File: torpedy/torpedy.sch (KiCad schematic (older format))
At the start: 45 parts, among them J1 Charger R.C., J10 żółty, J11 zielony, J12 różowy, J13 niebieski, J14 czerwony, J15 brązowy, J16 ekran, J2 step_up - Vin, J3 step_up - Vout, J4 Zasilanie Serwa, J5 Batt HP, J6 RPi I/O, J7 Trigger, J8 biały, J9 szary, Q1 Q_NPN_BCE, Q2 IRL2203N, Q3 Q_NPN_BCE, Q4 IRL2203N, U1 LTV-817, U2 LTV-817, U3 LTV-817, U4 LTV-817

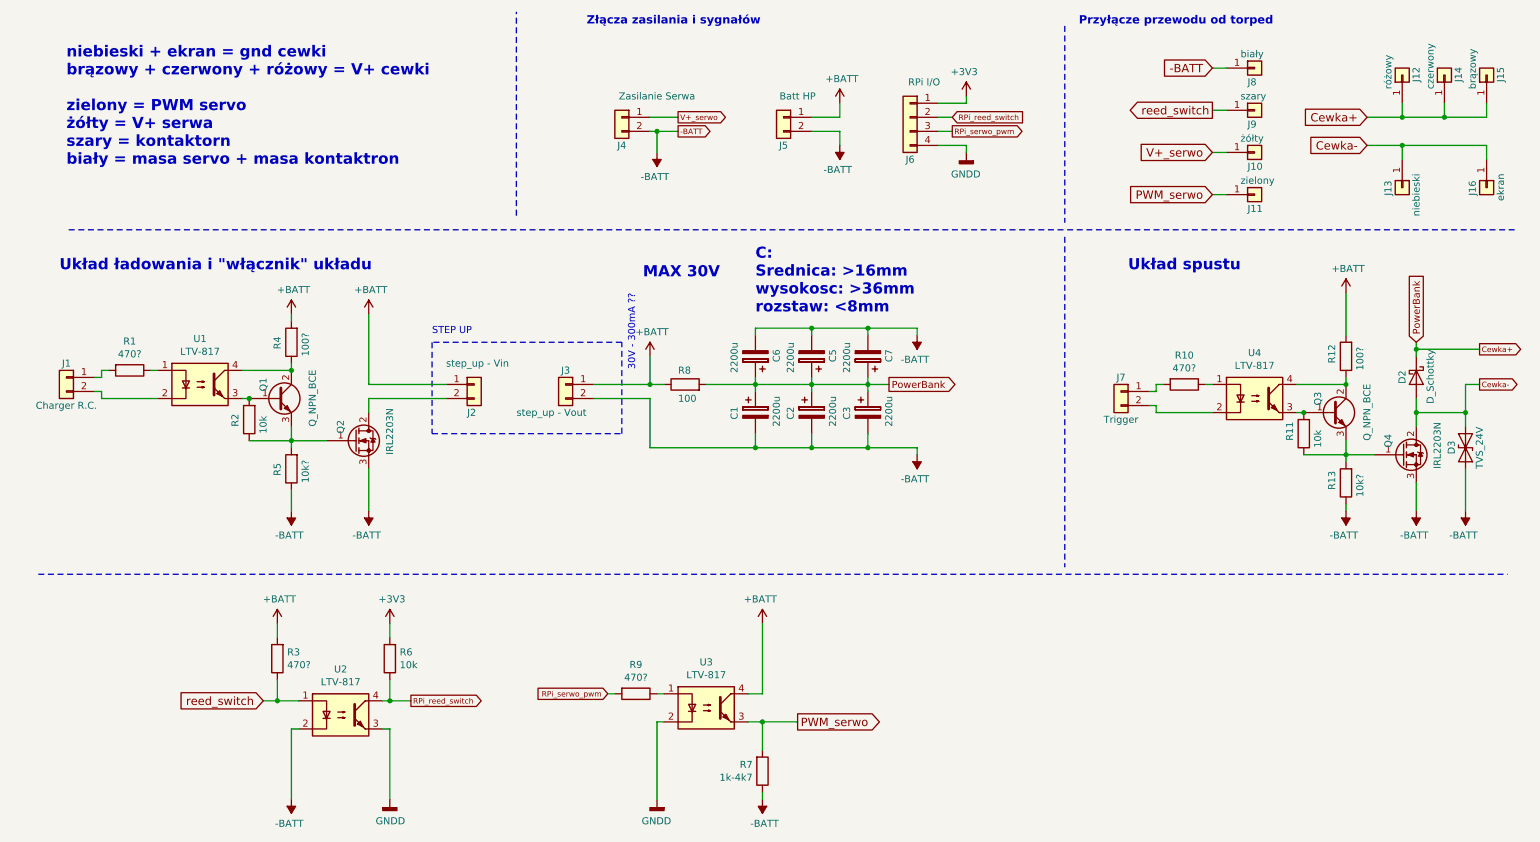
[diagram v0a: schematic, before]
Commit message: Jprdl nic nie umie i gupi jeste
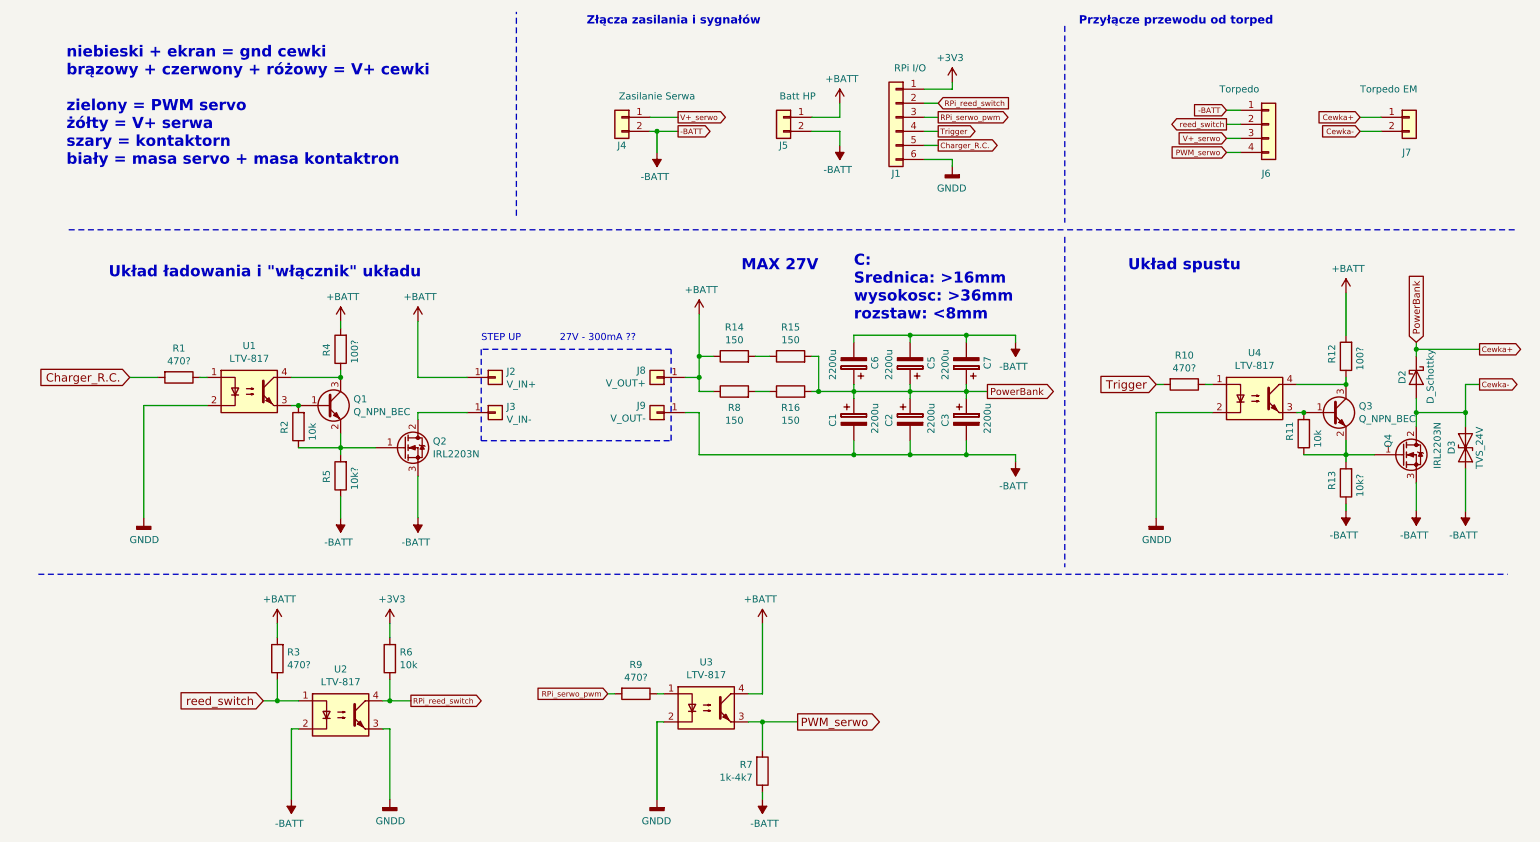
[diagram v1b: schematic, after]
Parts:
- removed J1: Charger R.C., symbol Connector_Generic:Conn_01x02
- removed J10: żółty, symbol Connector_Generic:Conn_01x01
- removed J11: zielony, symbol Connector_Generic:Conn_01x01
- removed J12: różowy, symbol Connector_Generic:Conn_01x01
- removed J13: niebieski, symbol Connector_Generic:Conn_01x01
- removed J14: czerwony, symbol Connector_Generic:Conn_01x01
- removed J15: brązowy, symbol Connector_Generic:Conn_01x01
- removed J16: ekran, symbol Connector_Generic:Conn_01x01
- removed J2: step_up - Vin, symbol Connector_Generic:Conn_01x02
- removed J3: step_up - Vout, symbol Connector_Generic:Conn_01x02
- removed Q1, Q3: Q_NPN_BCE, symbol Device:Q_NPN_BCE
- added J1: RPi I/O, Connector_Molex:Molex_SPOX_5267-06A_1x06_P2.50mm_Vertical, symbol Connector_Generic:Conn_01x06
- added J2: V_IN+, Connector_PinHeader_2.54mm:PinHeader_1x01_P2.54mm_Vertical, symbol Connector_Generic:Conn_01x01
- added J3: V_IN-, Connector_PinHeader_2.54mm:PinHeader_1x01_P2.54mm_Vertical, symbol Connector_Generic:Conn_01x01
- added Q1, Q3: Q_NPN_BEC, Package_TO_SOT_SMD:SOT-23_Handsoldering, symbol Device:Q_NPN_BEC
- added R14, R15, R16: 150, Resistor_THT:R_Axial_DIN0414_L11.9mm_D4.5mm_P20.32mm_Horizontal, symbol Device:R
- D2: footprint (none) -> Diode_SMD:D_SMC_Handsoldering
- D3: footprint (none) -> Diode_SMD:D_SMB_Handsoldering
- J4, J5: footprint (none) -> Connector_Molex:Molex_Mini-Fit_Jr_5566-02A_2x01_P4.20mm_Vertical
- J6: value RPi I/O -> Torpedo; footprint (none) -> Connector_Molex:Molex_SPOX_5267-04A_1x04_P2.50mm_Vertical
- J7: value Trigger -> Torpedo EM; footprint (none) -> Connector_Molex:Molex_Mini-Fit_Jr_5566-02A_2x01_P4.20mm_Vertical
- J8: value biały -> V_OUT+; footprint (none) -> Connector_PinHeader_2.54mm:PinHeader_1x01_P2.54mm_Vertical
- J9: value szary -> V_OUT-; footprint (none) -> Connector_PinHeader_2.54mm:PinHeader_1x01_P2.54mm_Vertical
- Q2, Q4: footprint (none) -> Package_TO_SOT_SMD:TO-263-2
- R1, R10, R11, R12, R13, R2, R3, R4, R5, R6, R7, R9: footprint (none) -> Resistor_SMD:R_0805_2012Metric_Pad1.15x1.40mm_HandSolder
- R8: value 100 -> 150; footprint (none) -> Resistor_THT:R_Axial_DIN0414_L11.9mm_D4.5mm_P20.32mm_Horizontal
- U1, U2, U3, U4: footprint Package_DIP:DIP-4_W7.62mm -> Package_DIP:SMDIP-4_W9.53mm
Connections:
- net +3V3: now also J1.1 (Pin_1); no longer J6.1 (Pin_1)
- net +BATT: now also J8.1 (Pin_1), J2.1 (Pin_1), R14.1
- net -BATT: now also J6.1 (Pin_1), J9.1 (Pin_1); no longer J8.1 (Pin_1)
- net Cewka+: now also J7.1 (Pin_1), R15.2, R16.2; no longer R8.2
- net Cewka-: now also J7.2 (Pin_2)
- net GNDD: now also U1.2, U4.2, J1.6 (Pin_6); no longer J6.4 (Pin_4)
- net PWM_serwo: now also J6.4 (Pin_4)
- net RPi_reed_switch: now also J1.2 (Pin_2); no longer J6.2 (Pin_2)
- net RPi_serwo_pwm: now also J1.3 (Pin_3); no longer J6.3 (Pin_3)
- net V+_serwo: now also J6.3 (Pin_3)
- net reed_switch: now also J6.2 (Pin_2); no longer J9.1 (Pin_1)
- net at Q4.1 (G), R11.1, R13.2: now also Q3.2 (E)
- net at R12.1, U4.4: now also Q3.3 (C)
- net at R11.2, U4.3: now also Q3.1 (B)
- net Trigger: now reaches R10.2
- net Trigger: now also J1.4 (Pin_4); no longer J7.1 (Pin_1)
- net at Q2.2 (D): now also J3.1 (Pin_1)
- net at Q2.1 (G), R2.1, R5.2: now also Q1.2 (E)
- net at R4.1, U1.4: now also Q1.3 (C)
- net at R2.2, U1.3: now also Q1.1 (B)
- net Charger_R.C.: now reaches R1.2
- net Charger_R.C.: now also J1.5 (Pin_5)
- new net: R16.1, R8.2
- new net: R14.2, R15.1
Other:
- note added: "27V - 300mA ??"
- note added: "MAX 27V"
- note removed: "30V - 300mA ??"
- note removed: "MAX 30V"
- moved on the sheet: C1, C2, C3, C5, C6, C7, Q2, R1, R2, R4, R5, R8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

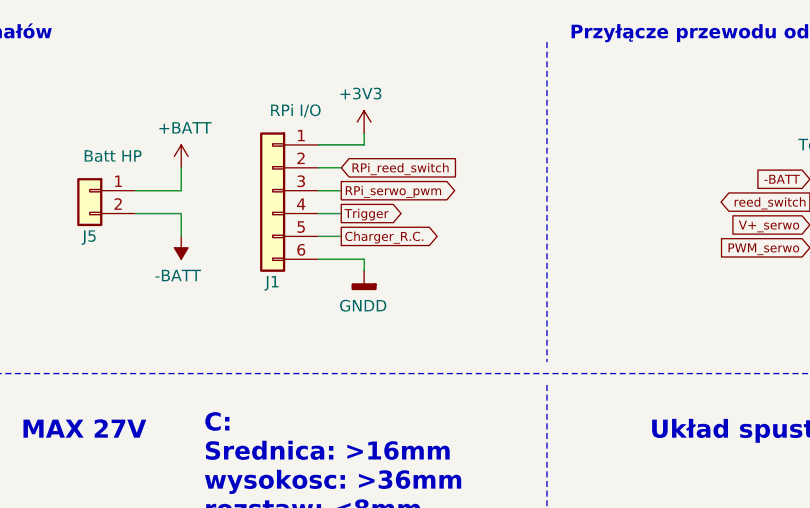
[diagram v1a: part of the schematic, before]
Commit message: Schemat pcb - początek
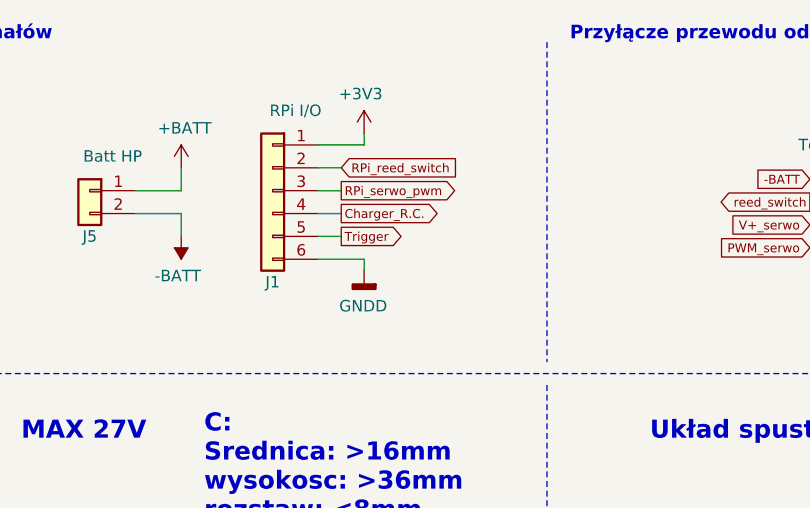
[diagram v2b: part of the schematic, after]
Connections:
- net Charger_R.C.: now also J1.4 (Pin_4); no longer J1.5 (Pin_5)
- net Trigger: now also J1.5 (Pin_5); no longer J1.4 (Pin_4)
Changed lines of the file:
@@
 EESchema Schematic File Version 4
 LIBS:torpedy-cache
-EELAYER 29 0
+EELAYER 26 0
 EELAYER END
 $Descr A4 11693 8268
@@
 Text GLabel 8500 3250 0    59   Input ~ 0
 Trigger
+Text GLabel 6950 1550 2    39   Output ~ 0
+Trigger
 Text GLabel 6950 1450 2    39   Output ~ 0
-Trigger
-Text GLabel 6950 1550 2    39   Output ~ 0
 Charger_R.C.
 $Comp
